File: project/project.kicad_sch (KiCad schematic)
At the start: 42 parts, among them J1 Conn_02x16_Odd_Even, J2 TYPE-C 6P(040新), SW1 SS-12D10L9, U1 DRV8833PWPR, U2 CH224K, U3 DRV8833PWPR, U4 AP63203WU-7, U5 TP4056, U6 AP2114, U7 MT3608L

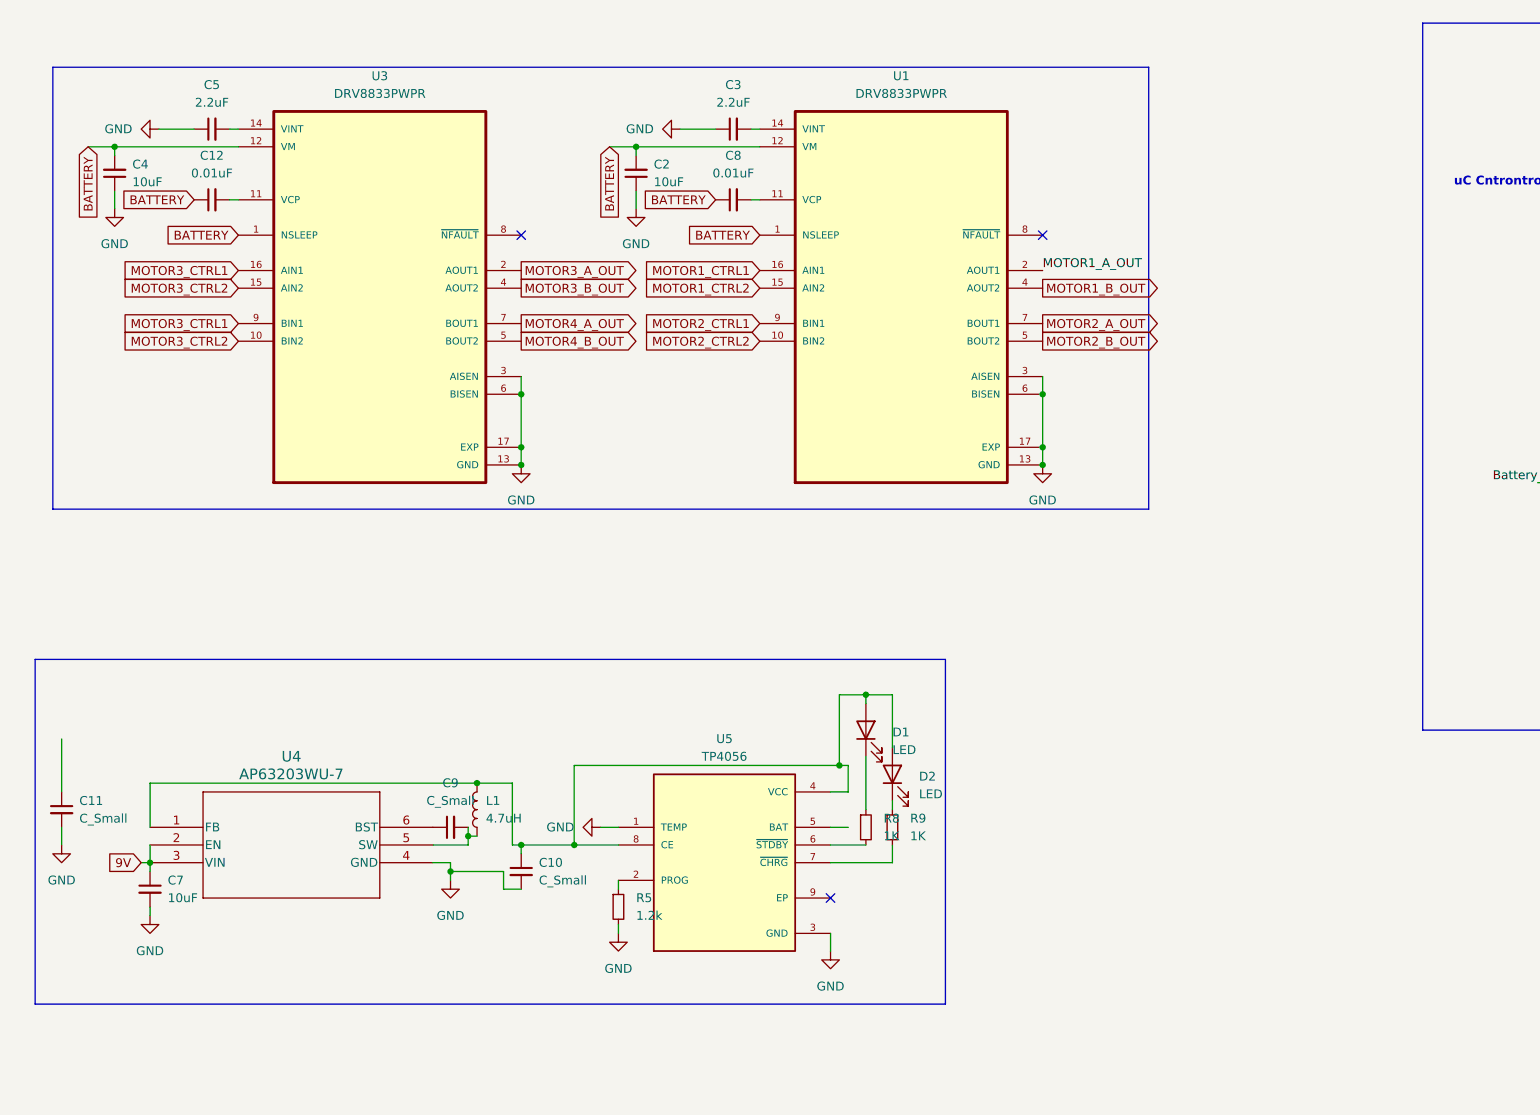
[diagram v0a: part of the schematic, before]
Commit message: NEW
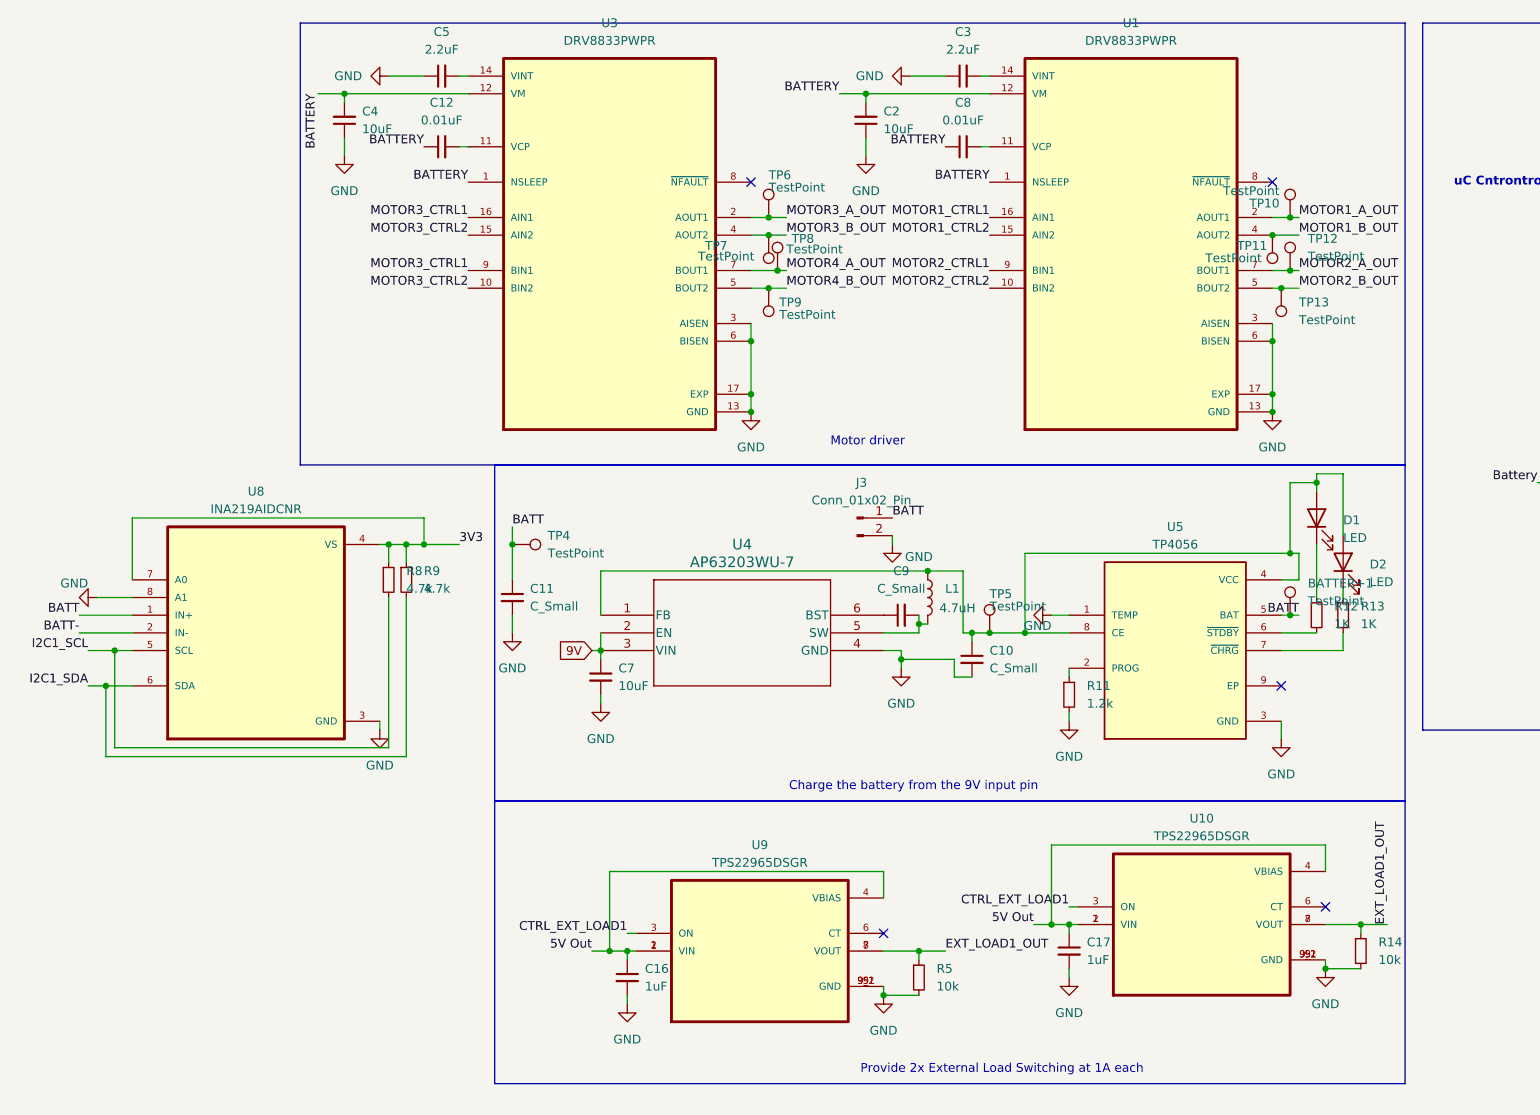
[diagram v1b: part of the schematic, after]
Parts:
- added BATTER+1, TP10, TP11, TP12, TP13, TP4, TP5, TP6, TP7, TP8, TP9: TestPoint, symbol Connector:TestPoint
- added C16, C17: 1uF, symbol Device:C_Small
- added J3: Conn_01x02_Pin, symbol Connector:Conn_01x02_Pin
- added R14, R5: 10k, symbol Device:R_Small
- added R8: 4.7k, Resistor_SMD:R_0402_1005Metric_Pad0.72x0.64mm_HandSolder, symbol Device:R_Small
- added R9: 4.7k, symbol Device:R_Small
- added U10, U9: TPS22965DSGR, TPS22965DSGR:SON50P200X200X80-9N, symbol TPS22965DSGR:TPS22965DSGR
- added U8: INA219AIDCNR, INA219AIDCNR:SOT65P280X145-8N, symbol INA219:INA219AIDCNR
- U1: LCSC (none) -> C50506
- renumbered R5 to R11, R8 to R12, R9 to R13
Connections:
- net 5V Out: now also C16.1, C17.1, U10.1 (VIN), U10.2 (VIN), U10.4 (VBIAS), U9.1 (VIN), U9.2 (VIN), U9.4 (VBIAS)
- net BATT: now also C11.1, U5.5 (BAT), BATTER+1.1, J3.1 (Pin_1), TP4.1, U8.1 (IN+)
- net CTRL_EXT_LOAD1: now also U10.3 (ON), U9.3 (ON)
- net EXT_LOAD1_OUT: now also R14.1, R5.1, U10.7 (VOUT), U10.8 (VOUT), U9.7 (VOUT), U9.8 (VOUT)
- net GND: now also C16.2, C17.2, J3.2 (Pin_2), R14.2, R5.2, U10.5 (GND), U10.9 (GND), U10.9_1 (GND), U10.9_2 (GND), U8.3 (GND), U8.8 (A1), U9.5 (GND), U9.9 (GND), U9.9_1 (GND), U9.9_2 (GND)
- net I2C1_SCL: now also R8.2, U8.5 (SCL)
- net I2C1_SDA: now also R9.2, U8.6 (SDA)
- net MOTOR1_A_OUT: now also TP10.1
- net MOTOR1_B_OUT: now also TP11.1
- net MOTOR2_A_OUT: now also TP12.1
- net MOTOR2_B_OUT: now also TP13.1
- net MOTOR3_A_OUT: now also TP6.1
- net MOTOR3_B_OUT: now also TP7.1
- net MOTOR4_A_OUT: now also TP8.1
- net MOTOR4_B_OUT: now also TP9.1
- net at C10.1, D1.2 (A), D2.2 (A)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: now also TP5.1
- new net 3V3: R8.1, R9.1, U8.4 (VS), U8.7 (A0)
- new net BATT-: U8.2 (IN-)
- no-connect marks 5 -> 7
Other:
- note added: "Charge the battery from the 9V input pin"
- note added: "Motor driver"
- note added: "Provide 2x External Load Switching at 1A each"
- moved on the sheet: C10, C11, C12, C2, C3, C4, C5, C7, C8, C9, D1, D2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

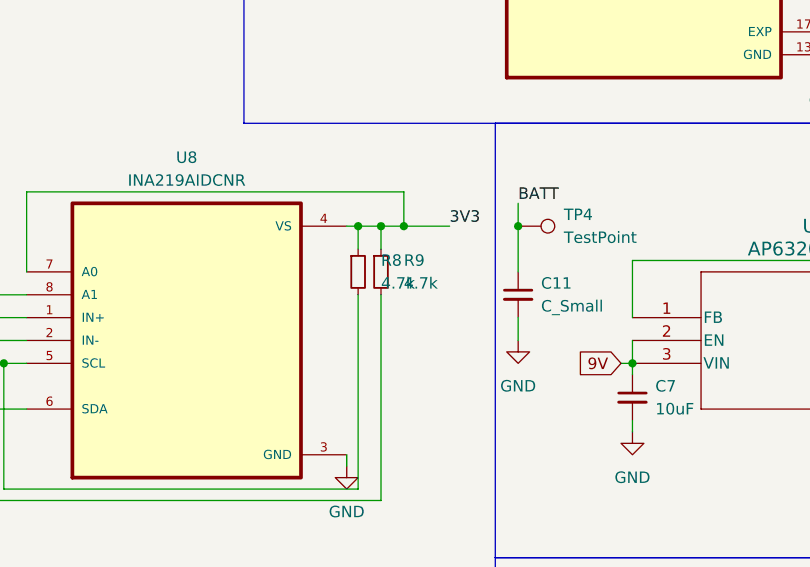
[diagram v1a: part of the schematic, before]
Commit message: CHANGED RESISTOR VALUE
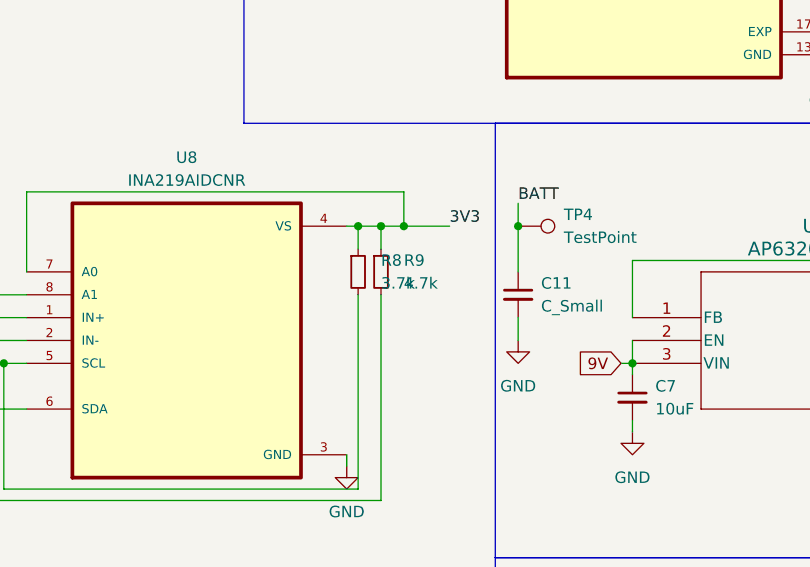
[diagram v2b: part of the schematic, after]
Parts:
- R8: value 4.7k -> 3.7k
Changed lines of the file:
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@@
 			)
 		)
-		(property "Value" "4.7k"
+		(property "Value" "3.7k"
 			(at 68.58 95.2499 0)
 			(effects
